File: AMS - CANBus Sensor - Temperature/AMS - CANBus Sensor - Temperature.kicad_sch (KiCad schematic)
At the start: 16 parts, among them J1 Power_And_CAN, J2 Power_And_CAN, J6 Screw_Terminal_01x02, Q1 IRF9Z34NPBF, U1 3568, U5 3568

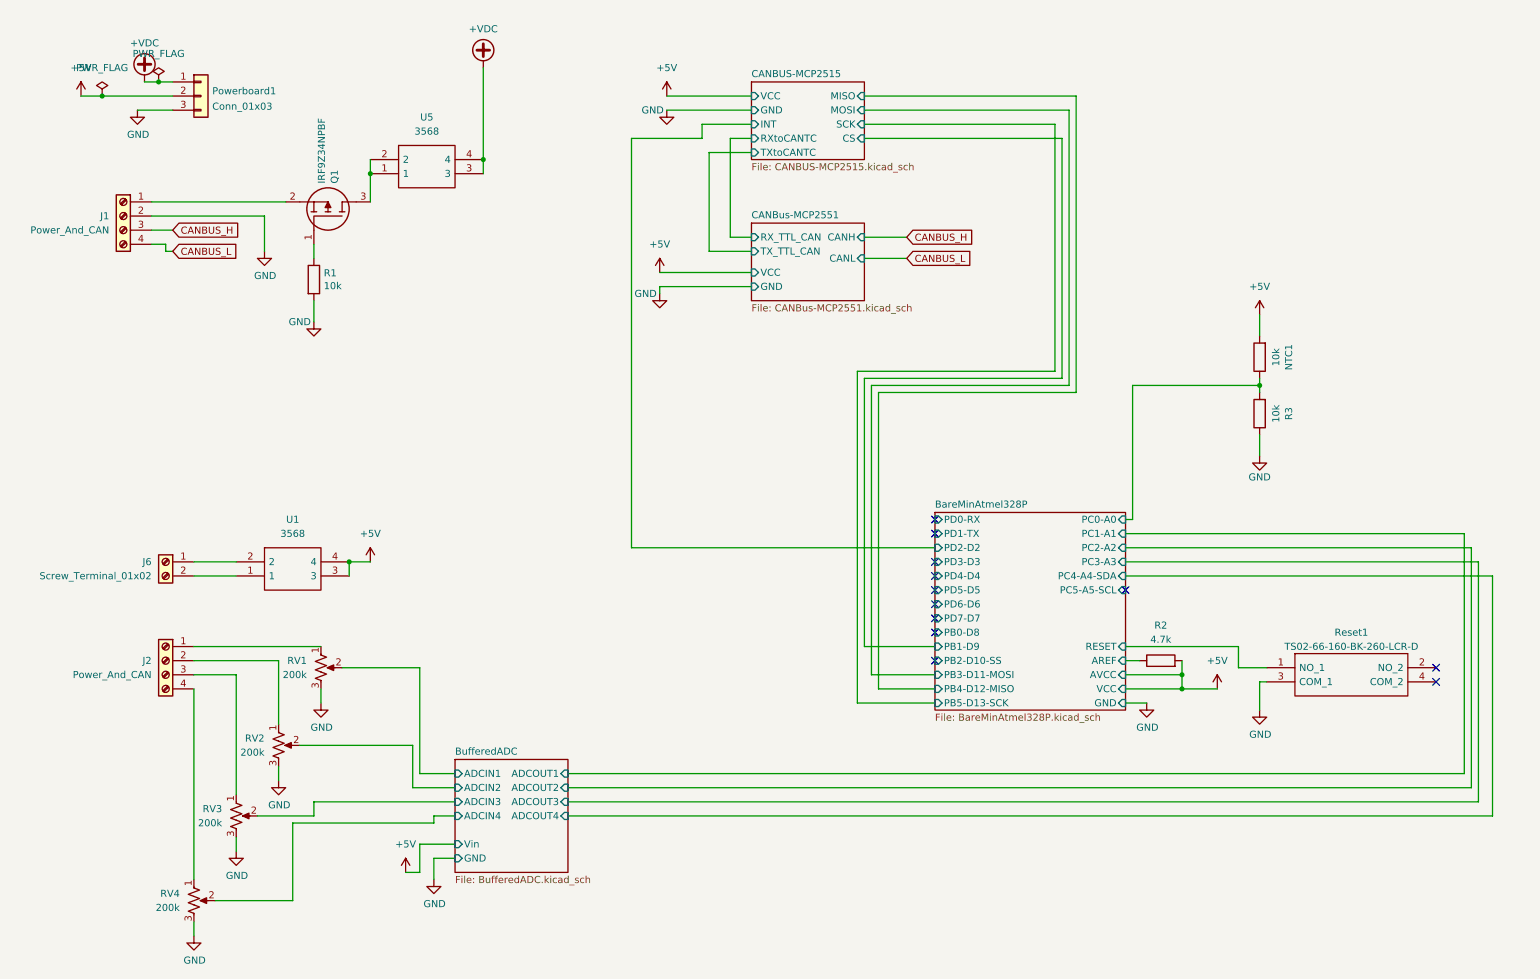
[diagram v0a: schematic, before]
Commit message: wip for the temp sensor
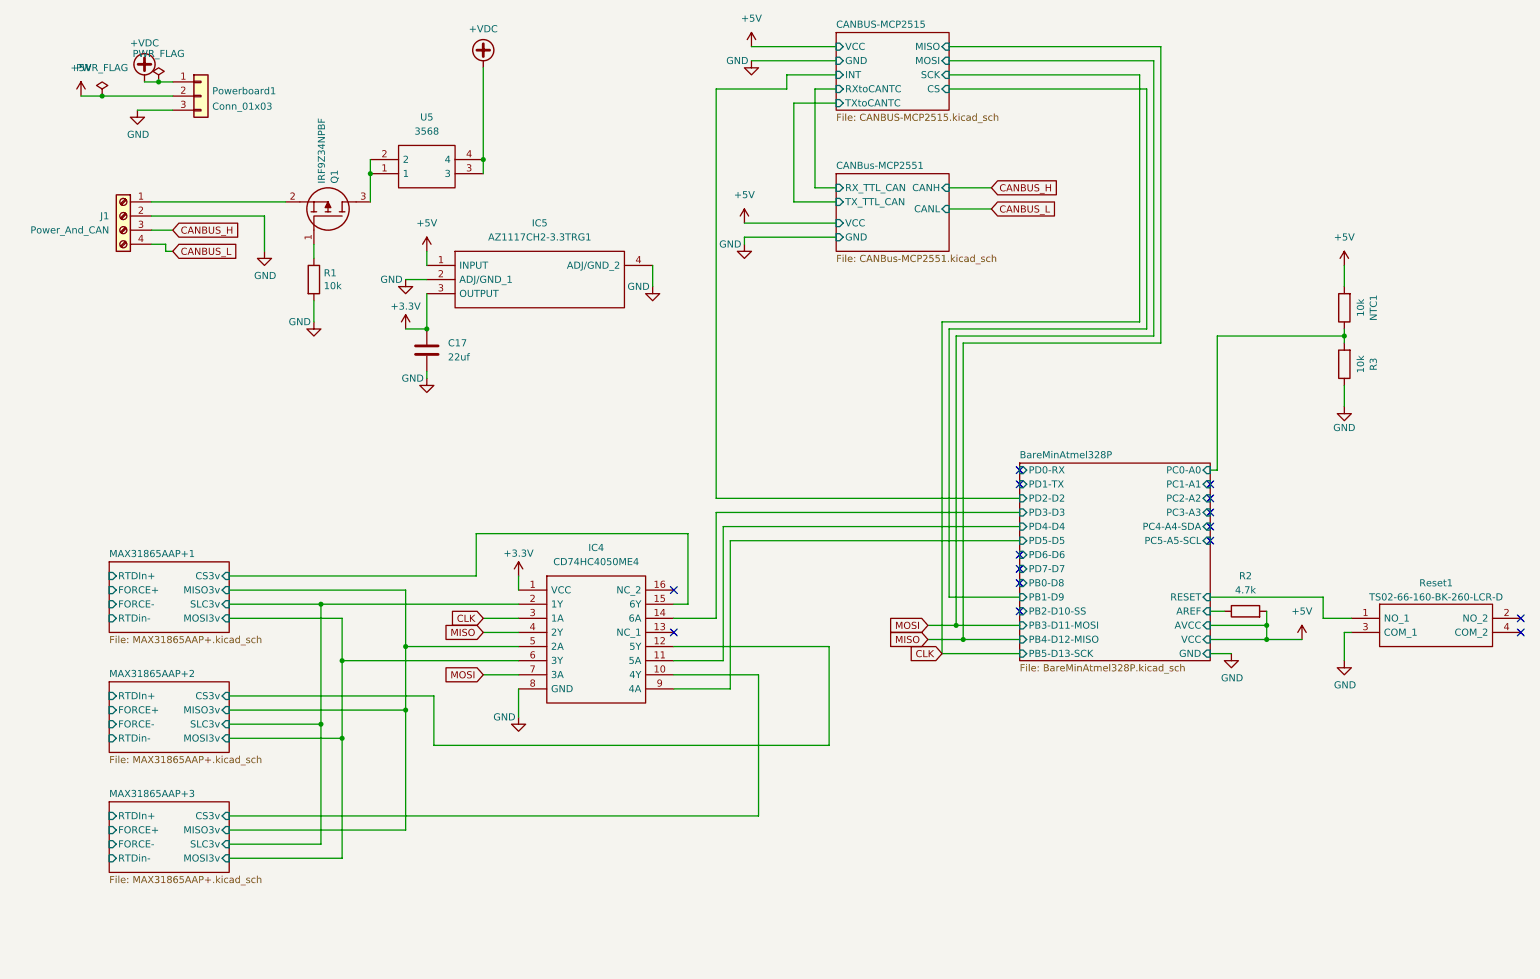
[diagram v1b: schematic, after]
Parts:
- removed J2: Power_And_CAN, TerminalBlock_Phoenix:TerminalBlock_Phoenix_MPT-0,5-4-2.54_1x04_P2.54mm_Horizontal, symbol Connector:Screw_Terminal_01x04
- removed J6: Screw_Terminal_01x02, TerminalBlock_Phoenix:TerminalBlock_Phoenix_MPT-0,5-2-2.54_1x02_P2.54mm_Horizontal, symbol Connector:Screw_Terminal_01x02
- removed RV1, RV2, RV3, RV4: 200k, Potentiometer_THT:Potentiometer_Bourns_3296W_Vertical, symbol Device:R_Potentiometer_US
- removed U1: 3568, 3568, symbol SamacSys_Parts:3568
- added C17: 22uf, Capacitor_SMD:C_1206_3216Metric_Pad1.33x1.80mm_HandSolder, symbol Device:C
- added IC4: CD74HC4050ME4, SOIC127P600X175-16N, symbol SamacSys_Parts:CD74HC4050ME4
- added IC5: AZ1117CH2-3.3TRG1, SOT230P700X180-4N, symbol SamacSys_Parts:AZ1117CH2-3.3TRG1
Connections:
- net +5V: now also IC5.1 (INPUT)
- net BareMinAtmel328P/PD3-D3: now also IC4.14 (6A)
- net BareMinAtmel328P/PD4-D4: now also IC4.11 (5A)
- net BareMinAtmel328P/PD5-D5: now also IC4.9 (4A)
- net GND: now also C17.1, IC4.8 (GND), IC5.2 (ADJ/GND_1), IC5.4 (ADJ/GND_2)
- new net +3.3V: C17.2, IC4.1 (VCC), IC5.3 (OUTPUT)
- new net CLK: IC4.3 (1A)
- new net MAX31865AAP+1/CS3v: IC4.15 (6Y)
- new net MAX31865AAP+1/MISO3v: IC4.5 (2A)
- new net MAX31865AAP+1/MOSI3v: IC4.6 (3Y)
- new net MAX31865AAP+1/SLC3v: IC4.2 (1Y)
- new net MAX31865AAP+2/CS3v: IC4.12 (5Y)
- new net MAX31865AAP+3/CS3v: IC4.10 (4Y)
- new net MISO: IC4.4 (2Y)
- new net MOSI: IC4.7 (3A)
- no-connect marks 12 -> 15
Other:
- removed sheet BufferedADC
- added sheet MAX31865AAP+1 (MAX31865AAP+.kicad_sch)
- added sheet MAX31865AAP+2 (MAX31865AAP+.kicad_sch)
- added sheet MAX31865AAP+3 (MAX31865AAP+.kicad_sch)
- moved on the sheet: NTC1, R2, R3, Reset1
